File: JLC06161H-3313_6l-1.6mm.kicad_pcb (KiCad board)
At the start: 6 copper layers, 24 x 24 mm, 0 parts

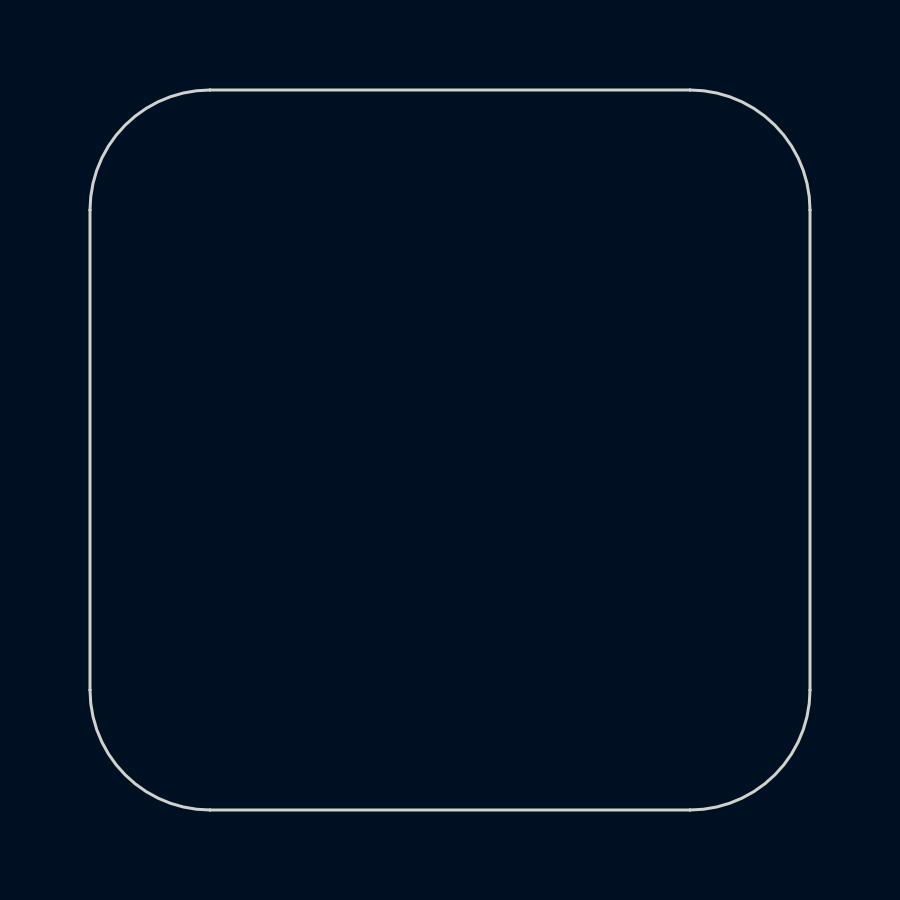
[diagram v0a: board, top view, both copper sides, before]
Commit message: add default zone
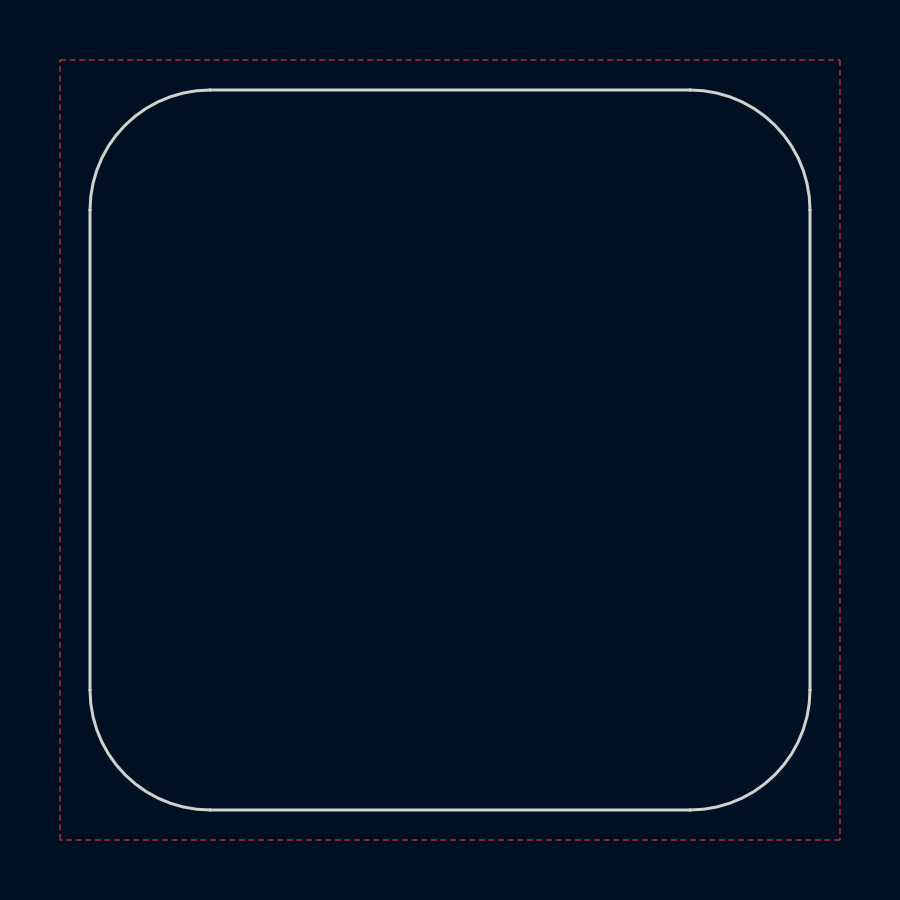
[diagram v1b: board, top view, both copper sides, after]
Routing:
- added copper zone on F.Cu, net (none)
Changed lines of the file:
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@@
 		(layer "Edge.Cuts")
 	)
+	(zone
+		(net 0)
+		(net_name "")
+		(layer "F.Cu")
+		(hatch edge 0.5)
+		(connect_pads
+			(clearance 0.127)
+		)
+		(min_thickness 0.127)
+		(filled_areas_thickness no)
+		(fill
+			(thermal_gap 0.127)
+			(thermal_bridge_width 0.5)
+			(smoothing fillet)
+			(radius 1)
+			(island_removal_mode 1)
+			(island_area_min 10)
+		)
+		(polygon
+			(pts
+				(xy 29 29) (xy 55 29) (xy 55 55) (xy 29 55)
+			)
+		)
+	)
 )

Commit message: update
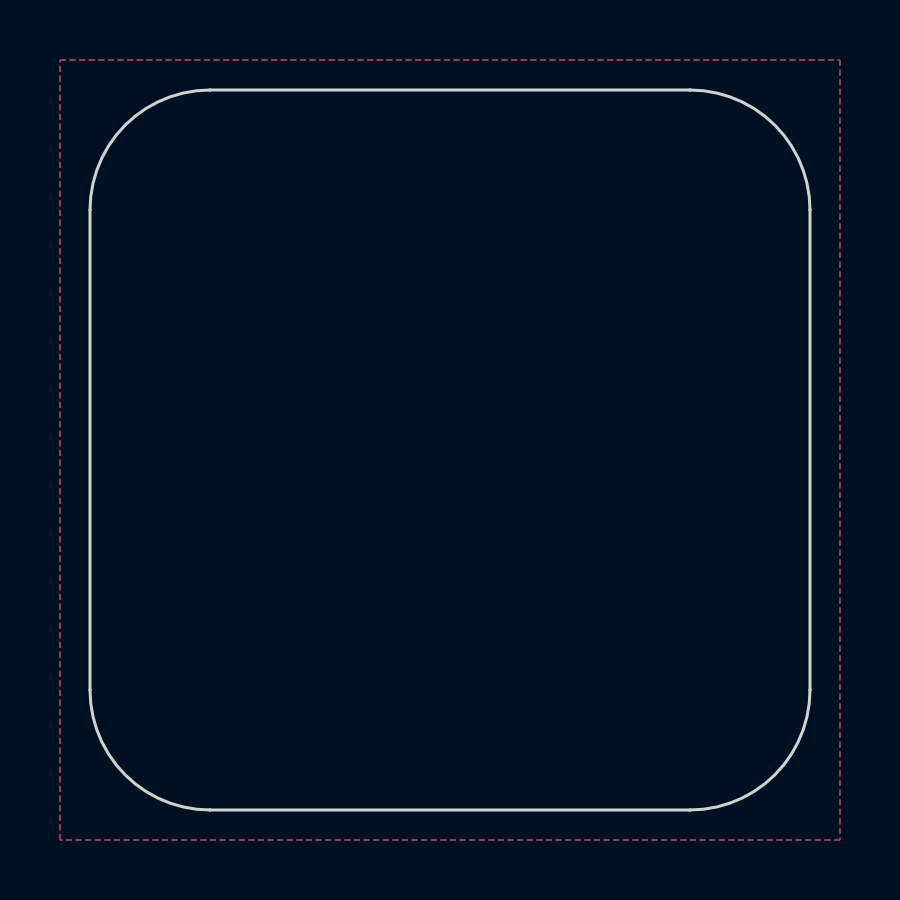
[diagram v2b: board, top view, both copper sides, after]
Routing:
- added copper zone on B.Cu, net (none)
- added copper zone on In1.Cu, net (none)
- added copper zone on In2.Cu, net (none)
- added copper zone on In3.Cu, net (none)
- added copper zone on In4.Cu, net (none)
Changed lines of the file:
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@@
 		(net 0)
 		(net_name "")
-		(layer "F.Cu")
+		(layers "F&B.Cu")
 		(hatch edge 0.5)
 		(connect_pads
@@
 			)
 		)
+	)
+	(zone
+		(net 0)
+		(net_name "")
+		(layers "In1.Cu" "In2.Cu" "In3.Cu" "In4.Cu")
+		(hatch edge 0.5)
+		(priority 1)
+		(connect_pads
+			(clearance 0.2)
+		)
+		(min_thickness 0.2)
+		(filled_areas_thickness no)
+		(fill
+			(thermal_gap 0.2)
+			(thermal_bridge_width 0.5)
+			(smoothing fillet)
+			(radius 1)
+			(island_removal_mode 1)
+			(island_area_min 10)
+		)
+		(polygon
+			(pts
+				(xy 28 28) (xy 56 28) (xy 56 56) (xy 28 56)
+			)
+		)
